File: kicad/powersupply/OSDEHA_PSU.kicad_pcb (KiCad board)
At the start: 2 copper layers, 104 parts, among them J1 340 VAC / 220 mA, J2 340 VAC / 220 mA, J3 420 VAC / 75 mA, J4 9 VAC / 4.5 A, J5 Stator bias, J6 HV-L, J7 HV-R, J8 HEATERS-LEFT, J9 HEATERS-RIGHT, K1 RT424006, Q1 BD138, Q10 BC550, Q11 LND150, Q12 LND150, Q13 NTHL1000N170M1, Q14 BC550, Q2 10M90S, Q3 LND150, Q4 LND150, Q5 NTHL1000N170M1, Q6 BC550, Q7 LND150, Q8 LND150, Q9 NTHL1000N170M1, U1 LM1085-ADJ, U2 NE555P

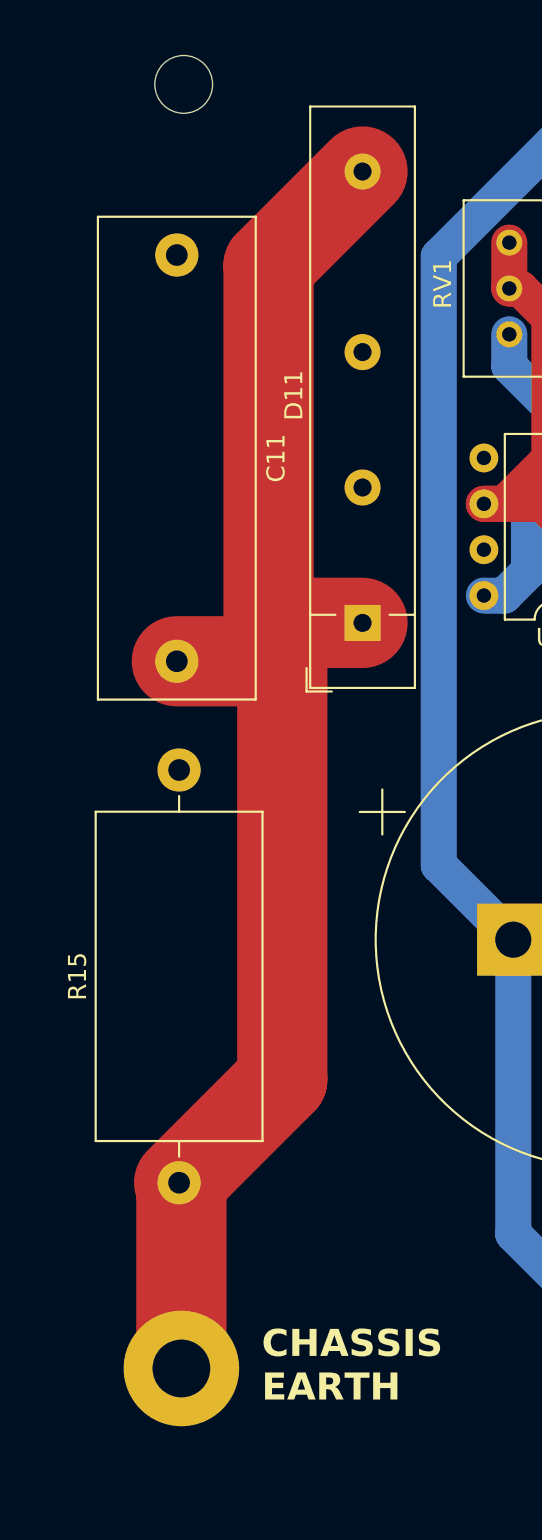
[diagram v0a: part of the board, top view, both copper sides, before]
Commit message: pcb psu
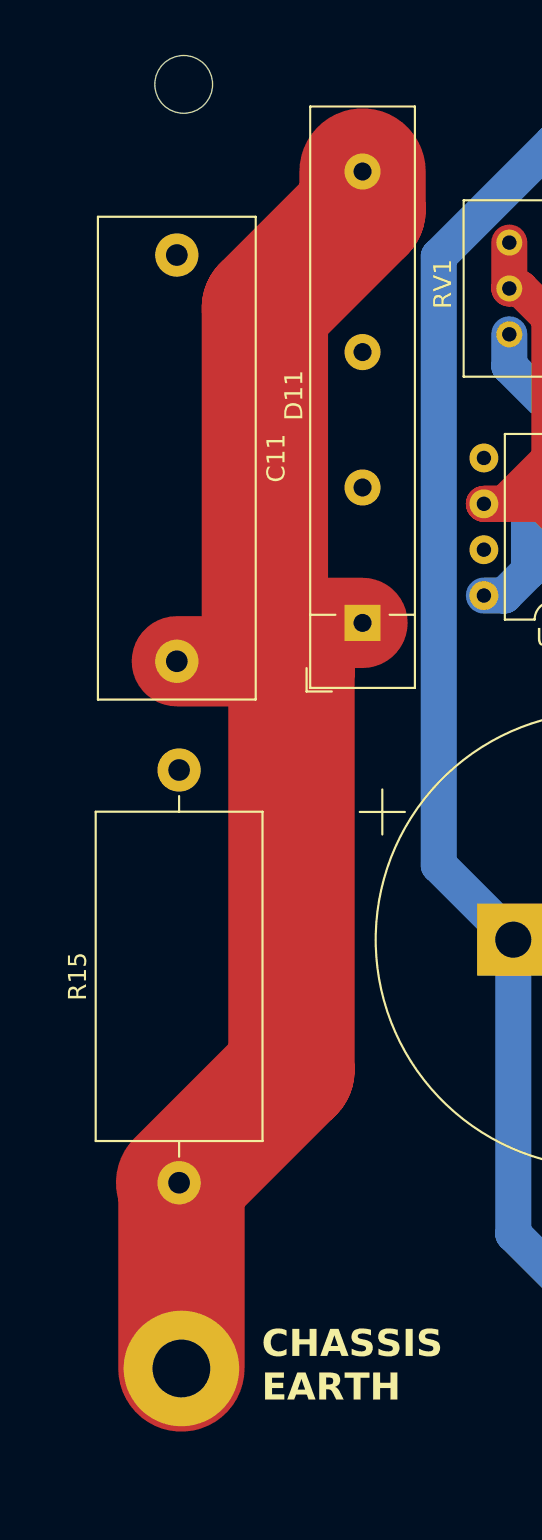
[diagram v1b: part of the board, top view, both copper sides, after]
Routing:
- net Earth_Protective: track 84.3 -> 84.9 mm
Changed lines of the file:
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@@
   (segment (start 252.309 84.407) (end 251.674 85.042) (width 2) (layer "B.Cu") (net 14))
   (segment (start 255.858 84.407) (end 252.309 84.407) (width 2) (layer "B.Cu") (net 14))
+  (segment (start 44.958 113.358) (end 44.958 135.509) (width 7) (layer "F.Cu") (net 15))
   (segment (start 43.688 112.088) (end 44.45 112.85) (width 5) (layer "F.Cu") (net 15))
-  (segment (start 44.45 136.017) (end 38.735 141.732) (width 5) (layer "F.Cu") (net 15))
-  (segment (start 48.895 85.725) (end 43.688 90.932) (width 5) (layer "F.Cu") (net 15))
+  (segment (start 44.45 112.85) (end 44.958 113.358) (width 7) (layer "F.Cu") (net 15))
+  (segment (start 43.4848 93.2688) (end 43.4848 111.8848) (width 7) (layer "F.Cu") (net 15))
+  (segment (start 48.895 85.725) (end 48.895 87.8586) (width 7) (layer "F.Cu") (net 15))
   (segment (start 38.862 141.859) (end 38.735 141.732) (width 2) (layer "F.Cu") (net 15))
-  (segment (start 38.862 152.019) (end 38.862 141.859) (width 5) (layer "F.Cu") (net 15))
+  (segment (start 38.862 152.019) (end 38.862 141.859) (width 7) (layer "F.Cu") (net 15))
+  (segment (start 44.958 135.509) (end 38.735 141.732) (width 7) (layer "F.Cu") (net 15))
   (segment (start 44.45 110.236) (end 44.45 112.85) (width 5) (layer "F.Cu") (net 15))
+  (segment (start 43.4848 111.8848) (end 43.688 112.088) (width 7) (layer "F.Cu") (net 15))
   (segment (start 38.608 112.85) (end 44.45 112.85) (width 5) (layer "F.Cu") (net 15))
-  (segment (start 44.45 112.85) (end 44.45 136.017) (width 5) (layer "F.Cu") (net 15))
-  (segment (start 43.688 90.932) (end 43.688 112.088) (width 5) (layer "F.Cu") (net 15))
+  (segment (start 48.895 87.8586) (end 43.4848 93.2688) (width 7) (layer "F.Cu") (net 15))
   (segment (start 44.939 110.725) (end 44.45 110.236) (width 2) (layer "F.Cu") (net 15))
   (segment (start 48.895 110.725) (end 44.939 110.725) (width 5) (layer "F.Cu") (net 15))

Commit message: psu pcb
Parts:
- moved R4 17.0 mm to (57.3, 144.5)
- moved H1 0.83 mm to (38.7, 81.7)
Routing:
- net Net-(D3-K): track 98.1 -> 86.9 mm
- net Net-(Q12-G): track 0.00 -> 5.76 mm
- net Net-(Q8-G): track 0.00 -> 5.76 mm
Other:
- board outline added: 239.3 x 78.3 mm
